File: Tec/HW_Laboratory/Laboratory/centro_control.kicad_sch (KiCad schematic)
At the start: 25 parts, among them J29 SPI, J31 BOT, J37 UART, J38 POWER, J39 USB_C_Receptacle_USB2.0_16P, SW1 BOOT, SW2 RESET, U23 ESP-12F, U24 AMS1117-3.3

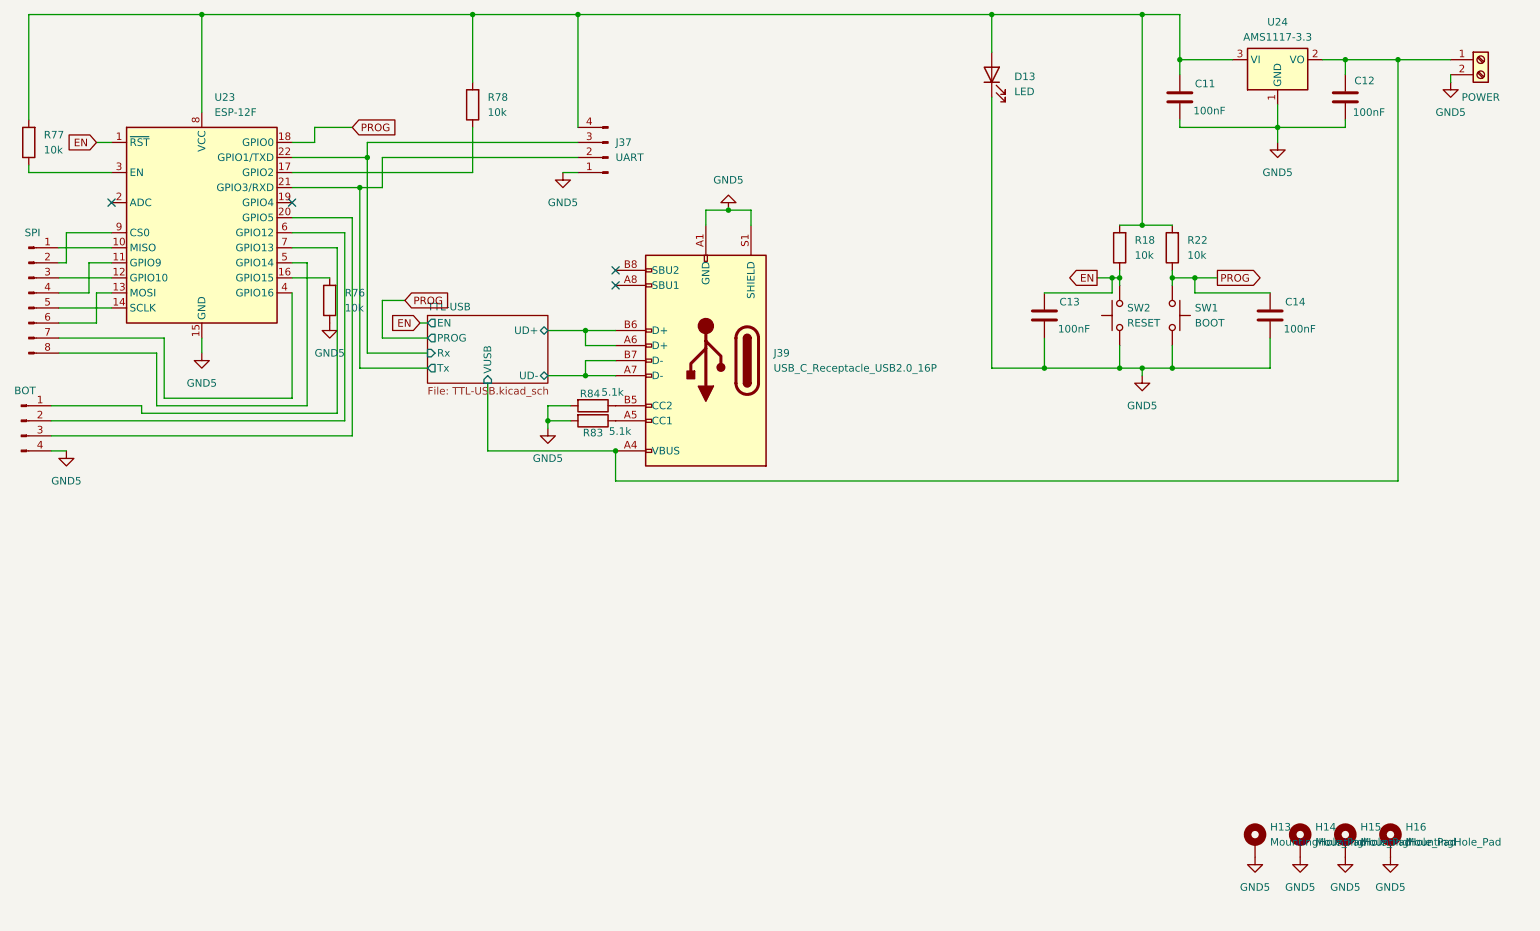
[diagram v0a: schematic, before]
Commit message: Laboratory v2.0:Update the PCB and the Software
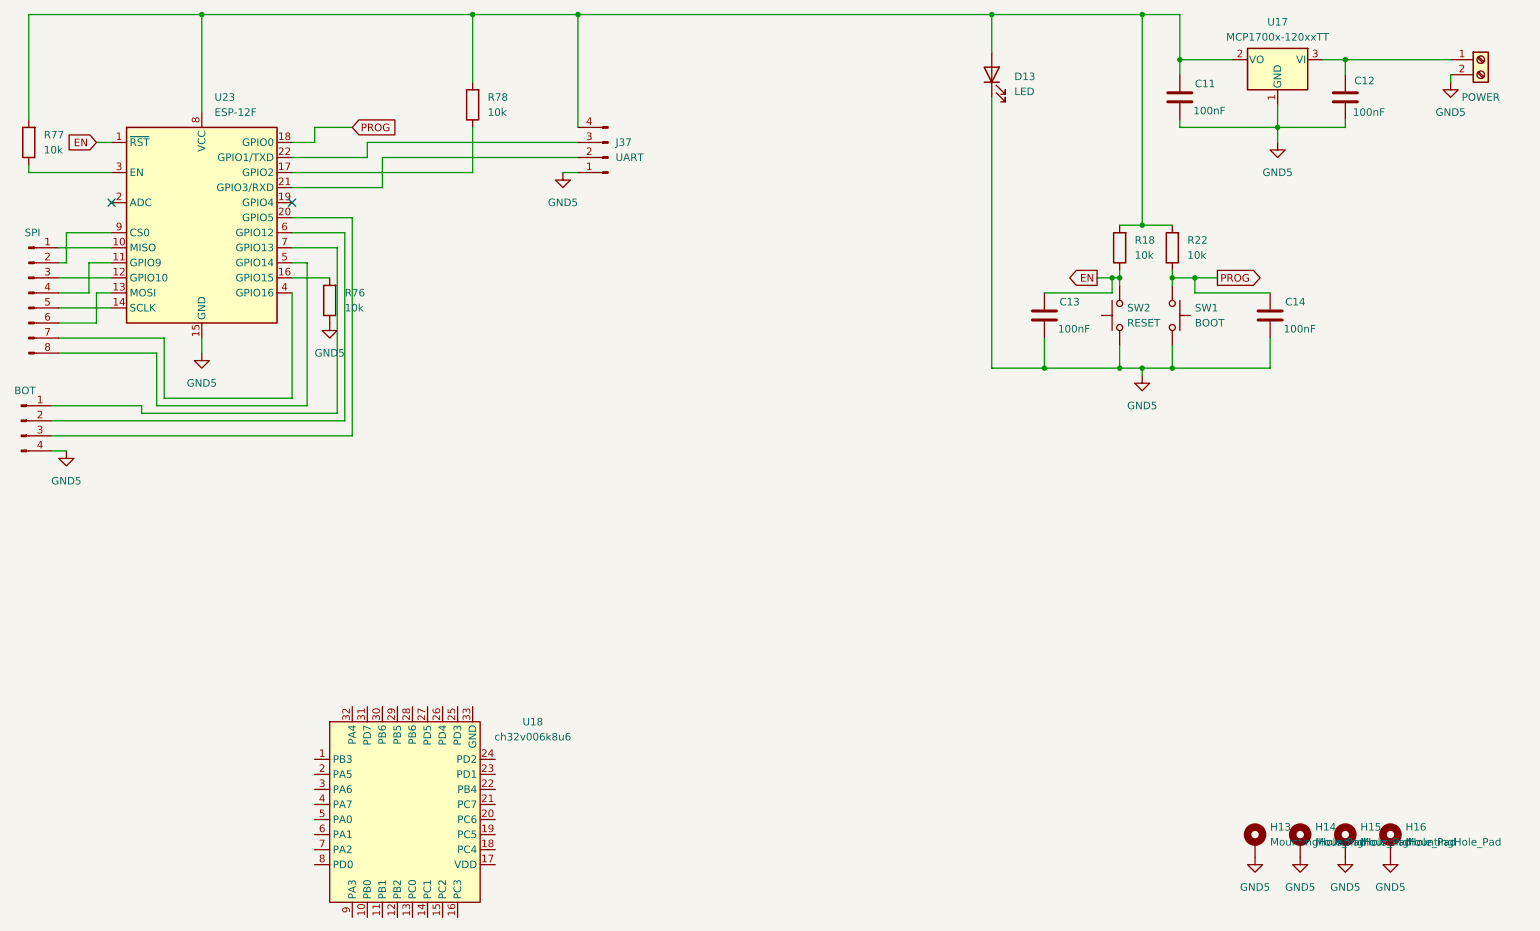
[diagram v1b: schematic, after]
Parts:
- removed J39: USB_C_Receptacle_USB2.0_16P, Connector_USB:USB_C_Receptacle_GCT_USB4105-xx-A_16P_TopMnt_Horizontal, symbol Connector:USB_C_Receptacle_USB2.0_16P
- removed R83, R84: 5.1k, Resistor_SMD:R_0603_1608Metric, symbol Device:R
- removed U24: AMS1117-3.3, Package_TO_SOT_SMD:SOT-223-3_TabPin2, symbol Regulator_Linear:AMS1117-3.3
- added U17: MCP1700x-120xxTT, Package_TO_SOT_SMD:SOT-23, symbol Regulator_Linear:MCP1700x-120xxTT
- added U18: ch32v006k8u6, Package_DFN_QFN:QFN-32-1EP_4x4mm_P0.4mm_EP2.65x2.65mm, symbol Custom:ch32v006k8u6
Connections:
- net GND5: now also U17.1 (GND)
- net at C11.1, D13.2 (A), J37.4 (Pin_4)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: now also U17.2 (VO)
- net TTL-USB/Rx: no longer names the net of J37.3 (Pin_3), U23.22 (GPIO1/TXD)
- net TTL-USB/Tx: no longer names the net of J37.2 (Pin_2), U23.21 (GPIO3/RXD)
- net TTL-USB/VUSB: no longer names the net of C12.1, J38.1 (Pin_1)
- net TTL-USB/VUSB: now also U17.3 (VI)
- no-connect marks 4 -> 2
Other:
- removed sheet TTL-USB
